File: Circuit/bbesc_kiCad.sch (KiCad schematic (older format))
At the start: 86 parts, among them J1 CONN_01X06, J2 CONN_01X06, J3 CONN_01X02, P1 CONN_01X06, P2 CONN_01X03, P3 CONN_01X04, P4 CONN_01X04, P5 CONN_01X01, P6 CONN_01X01, P7 CONN_01X01, Q1 Q_NMOS_GDS, Q2 Q_NMOS_GDS, Q3 Q_NMOS_GDS, Q4 Q_NMOS_GDS, Q5 Q_NMOS_GDS, Q6 Q_NMOS_GDS, U1 TJA1051T-SN65HVD230D, U2 teensy_3-2, U3 DRV_8302

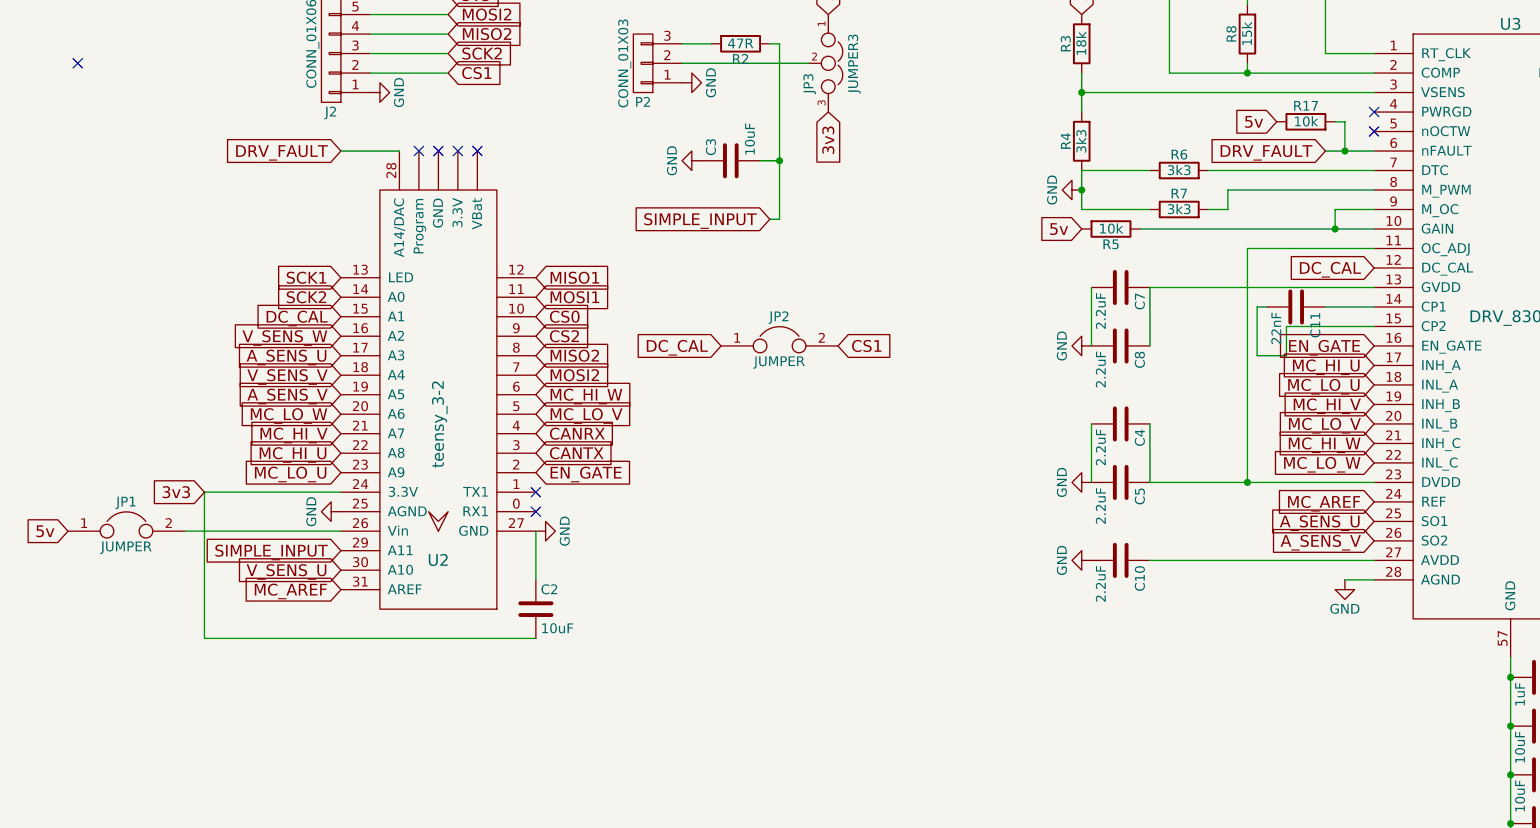
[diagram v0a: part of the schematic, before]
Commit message: rolling first PI loop :|
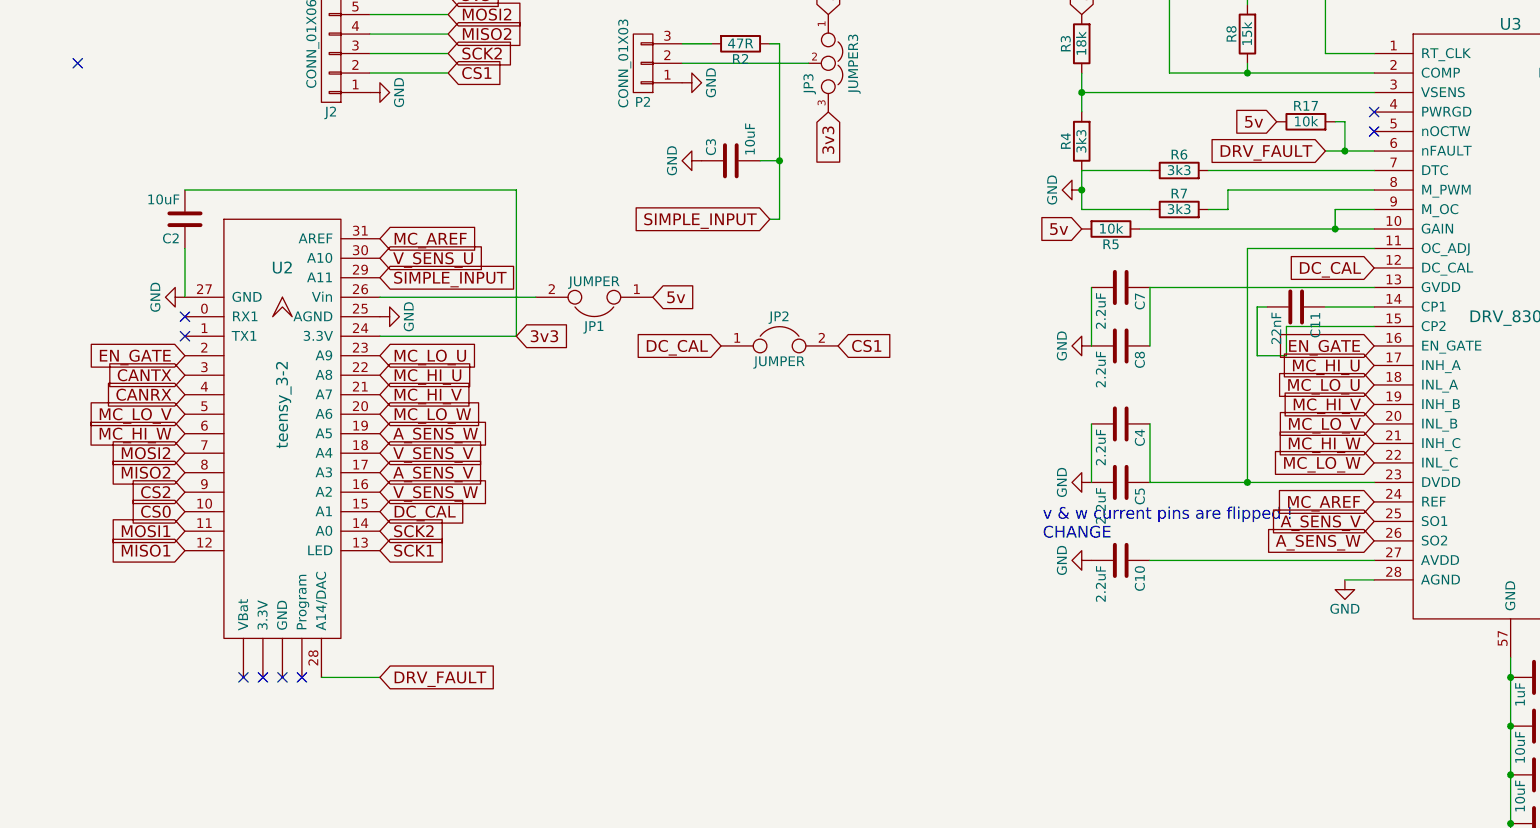
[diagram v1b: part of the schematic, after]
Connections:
- net A_SENS_U is gone; now on net A_SENS_V: U2.17 (A3), U3.25 (SO1)
- net A_SENS_V: no longer U2.19 (A5), U3.26 (SO2)
- new net A_SENS_W: U2.19 (A5), U3.26 (SO2)
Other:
- note added: "v & w current pins are flipped !\nCHANGE"
- moved on the sheet: C2, JP1, U2
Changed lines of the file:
@@
 	1    0    0    -1
 $EndComp
-Text GLabel 1650 7100 0    60   Input ~ 0
+Text GLabel 3250 6300 2    60   Input ~ 0
 3v3
 $Comp
@@
 Text GLabel 2900 4050 2    60   Input ~ 0
 SCK2
-Text GLabel 3350 6400 2    60   Input ~ 0
+Text GLabel 1550 7000 0    60   Input ~ 0
 MISO2
-Text GLabel 3350 6500 2    60   Input ~ 0
+Text GLabel 1550 6900 0    60   Input ~ 0
 MOSI2
-Text GLabel 2350 6100 0    60   Input ~ 0
+Text GLabel 2550 7300 2    60   Input ~ 0
 SCK2
-Text GLabel 3350 6300 2    60   Input ~ 0
+Text GLabel 1550 7100 0    60   Input ~ 0
 CS2
 $Comp
@@
 Text GLabel 4900 6350 2    60   Input ~ 0
 CS1
-Text GLabel 2350 6000 0    60   Input ~ 0
+Text GLabel 2550 7400 2    60   Input ~ 0
 SCK1
-NoConn ~ 3350 7100
-NoConn ~ 3350 7200
-NoConn ~ 3050 5350
-NoConn ~ 2950 5350
-NoConn ~ 2850 5350
-NoConn ~ 2750 5350
+NoConn ~ 1550 6300
+NoConn ~ 1550 6200
+NoConn ~ 1850 8050
+NoConn ~ 1950 8050
+NoConn ~ 2050 8050
+NoConn ~ 2150 8050
 $Comp
 L teensy_3-2 U2
 U 1 1 5915548A
-P 2850 6600
-F 0 "U2" H 2850 7450 60  0000 C CNN
-F 1 "teensy_3-2" V 2850 6750 60  0000 C CNN
-F 2 "teensy_3-2_bottomLess:Teensy3.2-bottomLess" H 2850 6750 60  0001 C CNN
-F 3 "" H 2850 6750 60  0001 C CNN
-	1    2850 6600
-	-1   0    0    1
+P 2050 6800
+F 0 "U2" H 2050 7650 60  0000 C CNN
+F 1 "teensy_3-2" V 2050 6950 60  0000 C CNN
+F 2 "teensy_3-2_bottomLess:Teensy3.2-bottomLess" H 2050 6950 60  0001 C CNN
+F 3 "" H 2050 6950 60  0001 C CNN
+	1    2050 6800
+	1    0    0    -1
 $EndComp
 $Comp
 L GND #PWR07
 U 1 1 59197249
-P 3350 7300
-F 0 "#PWR07" H 3350 7050 50  0001 C CNN
-F 1 "GND" H 3350 7150 50  0000 C CNN
-F 2 "" H 3350 7300 50  0001 C CNN
-F 3 "" H 3350 7300 50  0001 C CNN
-	1    3350 7300
-	0    -1   -1   0
+P 1550 6100
+F 0 "#PWR07" H 1550 5850 50  0001 C CNN
+F 1 "GND" H 1550 5950 50  0000 C CNN
+F 2 "" H 1550 6100 50  0001 C CNN
+F 3 "" H 1550 6100 50  0001 C CNN
+	1    1550 6100
+	0    1    1    0
 $EndComp
 Text GLabel 7650 6450 0    60   Input ~ 0
@@
 V_SENS_U
 Text GLabel 7650 7250 0    60   Input ~ 0
-A_SENS_U
+A_SENS_V
 Text GLabel 13450 2400 2    60   Input ~ 0
 PHASE_V
@@
 	1    0    0    -1
 $EndComp
-Text GLabel 2350 6700 0    60   Input ~ 0
+Text GLabel 2550 6700 2    60   Input ~ 0
 MC_LO_W
-Text GLabel 3350 6600 2    60   Input ~ 0
+Text GLabel 1550 6800 0    60   Input ~ 0
 MC_HI_W
-Text GLabel 3350 6700 2    60   Input ~ 0
+Text GLabel 1550 6700 0    60   Input ~ 0
 MC_LO_V
-Text GLabel 2350 6800 0    60   Input ~ 0
+Text GLabel 2550 6600 2    60   Input ~ 0
 MC_HI_V
-Text GLabel 2350 7000 0    60   Input ~ 0
+Text GLabel 2550 6400 2    60   Input ~ 0
 MC_LO_U
-Text GLabel 2350 6900 0    60   Input ~ 0
+Text GLabel 2550 6500 2    60   Input ~ 0
 MC_HI_U
-Text GLabel 2350 6400 0    60   Input ~ 0
-A_SENS_U
-Text GLabel 2350 7500 0    60   Input ~ 0
+Text GLabel 2550 7000 2    60   Input ~ 0
+A_SENS_V
+Text GLabel 2550 5900 2    60   Input ~ 0
 V_SENS_U
-Text GLabel 2350 6500 0    60   Input ~ 0
+Text GLabel 2550 6900 2    60   Input ~ 0
 V_SENS_V
-Text GLabel 2350 6600 0    60   Input ~ 0
-A_SENS_V
+Text GLabel 2550 6800 2    60   Input ~ 0
+A_SENS_W
 Text GLabel 7650 7350 0    60   Input ~ 0
-A_SENS_V
-Text GLabel 2350 6300 0    60   Input ~ 0
+A_SENS_W
+Text GLabel 2550 7100 2    60   Input ~ 0
 V_SENS_W
 $Comp
 L GND #PWR09
 U 1 1 5926BFB4
-P 2350 7200
-F 0 "#PWR09" H 2350 6950 50  0001 C CNN
-F 1 "GND" H 2350 7050 50  0000 C CNN
-F 2 "" H 2350 7200 50  0001 C CNN
-F 3 "" H 2350 7200 50  0001 C CNN
-	1    2350 7200
-	0    1    1    0
+P 2550 6200
+F 0 "#PWR09" H 2550 5950 50  0001 C CNN
+F 1 "GND" H 2550 6050 50  0000 C CNN
+F 2 "" H 2550 6200 50  0001 C CNN
+F 3 "" H 2550 6200 50  0001 C CNN
+	1    2550 6200
+	0    -1   -1   0
 $EndComp
 $Comp
@@
 Text GLabel 2900 4650 2    60   Input ~ 0
 MOSI2
-Text GLabel 3350 6100 2    60   Input ~ 0
+Text GLabel 1550 7300 0    60   Input ~ 0
 MOSI1
-Text GLabel 3350 6000 2    60   Input ~ 0
+Text GLabel 1550 7400 0    60   Input ~ 0
 MISO1
 $Comp
 L JUMPER JP1
 U 1 1 596F1F75
-P 1250 7300
-F 0 "JP1" H 1250 7450 50  0000 C CNN
-F 1 "JUMPER" H 1250 7220 50  0000 C CNN
-F 2 "Pin_Headers:Pin_Header_Straight_1x02_Pitch2.54mm" H 1250 7300 50  0001 C CNN
-F 3 "" H 1250 7300 50  0000 C CNN
-	1    1250 7300
-	1    0    0    -1
+P 3650 6100
+F 0 "JP1" H 3650 6250 50  0000 C CNN
+F 1 "JUMPER" H 3650 6020 50  0000 C CNN
+F 2 "Pin_Headers:Pin_Header_Straight_1x02_Pitch2.54mm" H 3650 6100 50  0001 C CNN
+F 3 "" H 3650 6100 50  0000 C CNN
+	1    3650 6100
+	-1   0    0    1
 $EndComp
 NoConn ~ 1000 4900
@@
 L C C2
 U 1 1 597222E7
-P 3350 7700
-F 0 "C2" H 3375 7800 50  0000 L CNN
-F 1 "10uF" H 3375 7600 50  0000 L CNN
-F 2 "Capacitors_SMD:C_1206_HandSoldering" H 3388 7550 50  0001 C CNN
-F 3 "" H 3350 7700 50  0001 C CNN
-	1    3350 7700
-	1    0    0    -1
+P 1550 5700
+F 0 "C2" H 1575 5800 50  0000 L CNN
+F 1 "10uF" H 1575 5600 50  0000 L CNN
+F 2 "Capacitors_SMD:C_1206_HandSoldering" H 1588 5550 50  0001 C CNN
+F 3 "" H 1550 5700 50  0001 C CNN
+	1    1550 5700
+	-1   0    0    1
 $EndComp
 $Comp
@@
 Text GLabel 4850 5150 3    60   Input ~ 0
 3v3
-Text GLabel 3350 6200 2    60   Input ~ 0
+Text GLabel 1550 7200 0    60   Input ~ 0
 CS0
 $Comp
@@
 	1    0    0    -1
 $EndComp
-Text GLabel 3350 6900 2    60   Input ~ 0
+Text GLabel 1550 6500 0    60   Input ~ 0
 CANTX
-Text GLabel 3350 6800 2    60   Input ~ 0
+Text GLabel 1550 6600 0    60   Input ~ 0
 CANRX
 Text GLabel 2250 1650 0    60   Input ~ 0
@@
 	1    0    0    -1
 $EndComp
-Text GLabel 950  7300 0    60   Input ~ 0
+Text GLabel 3950 6100 2    60   Input ~ 0
 5v
 Text GLabel 4850 4650 1    60   Input ~ 0
@@
 Text GLabel 4550 5700 0    60   Input ~ 0
 SIMPLE_INPUT
-Text GLabel 2350 7400 0    60   Input ~ 0
+Text GLabel 2550 6000 2    60   Input ~ 0
 SIMPLE_INPUT
 Text GLabel 10850 2200 0    60   Input ~ 0
@@
 Text GLabel 7650 6350 0    60   Input ~ 0
 EN_GATE
-Text GLabel 3350 7000 2    60   Input ~ 0
+Text GLabel 1550 6400 0    60   Input ~ 0
 EN_GATE
-Text GLabel 2350 7600 0    60   Input ~ 0
+Text GLabel 2550 5800 2    60   Input ~ 0
 MC_AREF
 $Comp
@@
 Text GLabel 7400 5350 0    60   Input ~ 0
 DRV_FAULT
-Text GLabel 2350 5350 0    60   Input ~ 0
+Text GLabel 2550 8050 2    60   Input ~ 0
 DRV_FAULT
 $Comp
@@
 Text GLabel 6150 5750 0    60   Input ~ 0
 5v
-Text GLabel 2350 6200 0    60   Input ~ 0
+Text GLabel 2550 7200 2    60   Input ~ 0
 DC_CAL
 Text HLabel 14950 3300 0    60   Input ~ 0
@@
 H_V_LO
 Wire Wire Line
-	1650 7100 2350 7100
+	3250 6300 2550 6300
 Wire Wire Line
 	2500 4550 2900 4550
@@
 	2500 4750 2900 4750
 Wire Wire Line
-	1550 7300 2350 7300
-Wire Wire Line
-	3350 7550 3350 7300
-Wire Wire Line
-	1650 7100 1650 7850
-Wire Wire Line
-	1650 7850 3350 7850
+	3350 6100 2550 6100
+Wire Wire Line
+	1550 5850 1550 6100
+Wire Wire Line
+	3250 6300 3250 5550
+Wire Wire Line
+	3250 5550 1550 5550
 Wire Wire Line
 	2500 2950 2900 2950
@@
 Connection ~ 7400 4250
 Wire Wire Line
-	2350 5350 2650 5350
+	2550 8050 2250 8050
 Wire Wire Line
 	7650 5050 6150 5050
@@
 Text GLabel 14550 7100 0    60   Input ~ 0
 PHASE_W
+Text Notes 5950 7350 0    60   ~ 0
+v & w current pins are flipped !\nCHANGE
 $EndSCHEMATC
